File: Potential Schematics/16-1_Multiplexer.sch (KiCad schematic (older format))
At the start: 2 parts, among them U181 74LS04, U194 74LS04

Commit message: Adding Multiply Devide
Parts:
- U181, U194: symbol 74LS04 -> 4-bit_processor-rescue:74LS04
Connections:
- net 5:1_AND/b is gone; now on net 5:1_AND/b: U194.2
- net 5:1_AND/c is gone; now on net 5:1_AND/c: U181.13
- net 5:1_AND/b: no longer U194.1
- net 5:1_AND/c: no longer U181.12, U181.8
- new net 5:1_AND/b: U194.1
- new net 5:1_AND/c: U181.12, U181.8
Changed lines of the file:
@@
-EESchema Schematic File Version 2
-LIBS:power
-LIBS:device
-LIBS:switches
-LIBS:relays
-LIBS:motors
-LIBS:transistors
-LIBS:conn
-LIBS:linear
-LIBS:regul
-LIBS:74xx
-LIBS:cmos4000
-LIBS:adc-dac
-LIBS:memory
-LIBS:xilinx
-LIBS:microcontrollers
-LIBS:dsp
-LIBS:microchip
-LIBS:analog_switches
-LIBS:motorola
-LIBS:texas
-LIBS:intel
-LIBS:audio
-LIBS:interface
-LIBS:digital-audio
-LIBS:philips
-LIBS:display
-LIBS:cypress
-LIBS:siliconi
-LIBS:opto
-LIBS:atmel
-LIBS:contrib
-LIBS:valves
+EESchema Schematic File Version 4
 LIBS:4-bit_processor-cache
-EELAYER 25 0
+EELAYER 26 0
 EELAYER END
 $Descr A4 11693 8268
 encoding utf-8
-Sheet 378 449
+Sheet 378 451
 Title "16:1 Multiplexer"
 Date "2018-09-14"
@@
 $EndSheet
 $Comp
-L 74LS04 U194
+L 4-bit_processor-rescue:74LS04 U194
 U 1 1 5BB53D19
 P 1700 5450
@@
 $EndComp
 $Comp
-L 74LS04 U181
+L 4-bit_processor-rescue:74LS04 U181
 U 6 1 5BB54417
 P 1400 5450
@@
 $EndComp
 $Comp
-L 74LS04 U181
+L 4-bit_processor-rescue:74LS04 U181
 U 5 1 5BB55464
 P 1100 5450
@@
 $EndComp
 $Comp
-L 74LS04 U181
+L 4-bit_processor-rescue:74LS04 U181
 U 4 1 5BB5546A
 P 800 5450

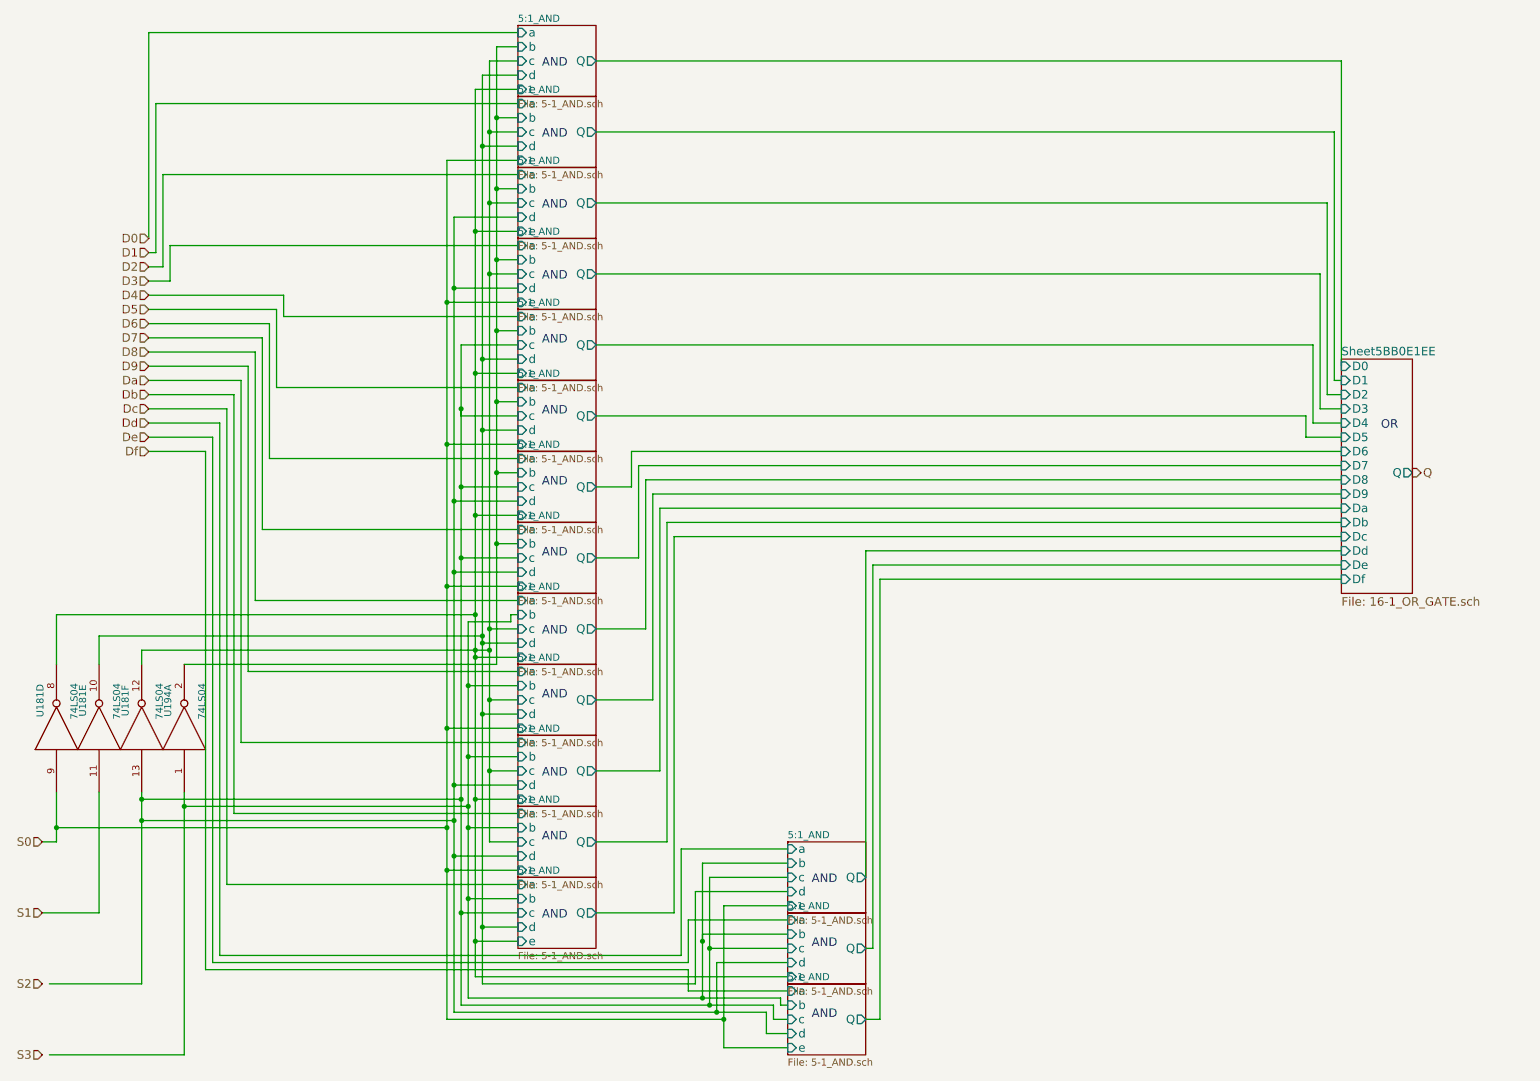
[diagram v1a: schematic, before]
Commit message: Finished PCB
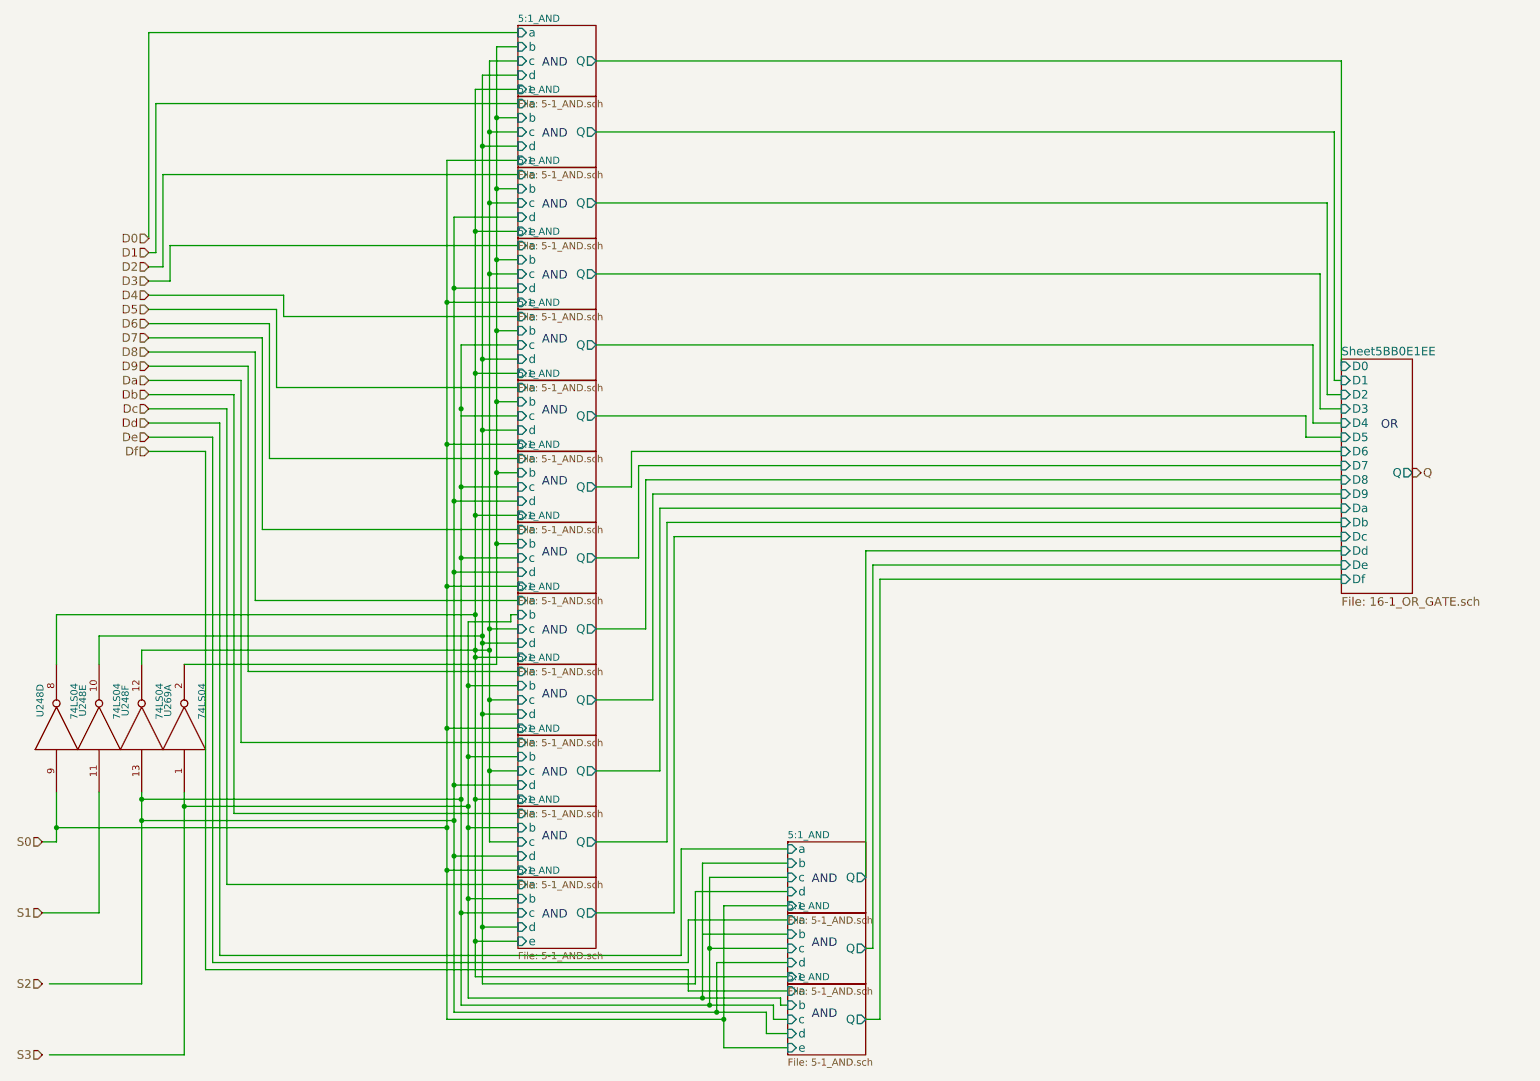
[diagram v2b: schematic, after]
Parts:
- U195: renamed from U181; footprint (none) -> Daniel_Kopp:DIP-14_300_ELL
- U208: renamed from U194; footprint (none) -> Daniel_Kopp:DIP-14_300_ELL
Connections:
- net 5:1_AND/b is gone; now on net 5:1_AND/b: U208.2
- net 5:1_AND/c is gone; now on net 5:1_AND/c: U195.13
- net 5:1_AND/b: no longer U208.1
- net 5:1_AND/c: no longer U195.12, U195.8
- new net 5:1_AND/b: U208.1
- new net 5:1_AND/c: U195.12, U195.8
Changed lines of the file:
@@
 $Descr A4 11693 8268
 encoding utf-8
-Sheet 378 451
+Sheet 378 456
 Title "16:1 Multiplexer"
 Date "2018-09-14"
@@
 $EndSheet
 $Comp
-L 4-bit_processor-rescue:74LS04 U194
+L 4-bit_processor-rescue:74LS04 U208
 U 1 1 5BB53D19
 P 1700 5450
-AR Path="/5B9D167A/5B9C0EA0/5BAE2F4B/5BAE3D50/5BB53D19" Ref="U194"  Part="1"
-AR Path="/5B9D167A/5B9C0EA0/5BAE2F4B/5BC8C0A9/5BB53D19" Ref="U194"  Part="5"
-AR Path="/5B9D167A/5B9C0EA0/5BAE2F4B/5BC8F4EC/5BB53D19" Ref="U233"  Part="3"
-AR Path="/5B9D167A/5B9C0EA0/5BAE2F4B/5BC8F503/5BB53D19" Ref="U253"  Part="1"
-F 0 "U194" H 1895 5565 50  0000 C CNN
+AR Path="/5B9D167A/5B9C0EA0/5BAE2F4B/5BAE3D50/5BB53D19" Ref="U208"  Part="1"
+AR Path="/5B9D167A/5B9C0EA0/5BAE2F4B/5BC8C0A9/5BB53D19" Ref="U208"  Part="5"
+AR Path="/5B9D167A/5B9C0EA0/5BAE2F4B/5BC8F4EC/5BB53D19" Ref="U248"  Part="3"
+AR Path="/5B9D167A/5B9C0EA0/5BAE2F4B/5BC8F503/5BB53D19" Ref="U269"  Part="1"
+F 0 "U269" H 1895 5565 50  0000 C CNN
 F 1 "74LS04" H 1890 5325 50  0000 C CNN
-F 2 "" H 1700 5450 50  0001 C CNN
+F 2 "Daniel_Kopp:DIP-14_300_ELL" H 1700 5450 50  0001 C CNN
 F 3 "" H 1700 5450 50  0001 C CNN
 	1    1700 5450
@@
 $EndComp
 $Comp
-L 4-bit_processor-rescue:74LS04 U181
+L 4-bit_processor-rescue:74LS04 U195
 U 6 1 5BB54417
 P 1400 5450
-AR Path="/5B9D167A/5B9C0EA0/5BAE2F4B/5BAE3D50/5BB54417" Ref="U181"  Part="6"
-AR Path="/5B9D167A/5B9C0EA0/5BAE2F4B/5BC8C0A9/5BB54417" Ref="U194"  Part="4"
-AR Path="/5B9D167A/5B9C0EA0/5BAE2F4B/5BC8F4EC/5BB54417" Ref="U233"  Part="2"
-AR Path="/5B9D167A/5B9C0EA0/5BAE2F4B/5BC8F503/5BB54417" Ref="U233"  Part="6"
-F 0 "U181" H 1595 5565 50  0000 C CNN
+AR Path="/5B9D167A/5B9C0EA0/5BAE2F4B/5BAE3D50/5BB54417" Ref="U195"  Part="6"
+AR Path="/5B9D167A/5B9C0EA0/5BAE2F4B/5BC8C0A9/5BB54417" Ref="U208"  Part="4"
+AR Path="/5B9D167A/5B9C0EA0/5BAE2F4B/5BC8F4EC/5BB54417" Ref="U248"  Part="2"
+AR Path="/5B9D167A/5B9C0EA0/5BAE2F4B/5BC8F503/5BB54417" Ref="U248"  Part="6"
+F 0 "U248" H 1595 5565 50  0000 C CNN
 F 1 "74LS04" H 1590 5325 50  0000 C CNN
-F 2 "" H 1400 5450 50  0001 C CNN
+F 2 "Daniel_Kopp:DIP-14_300_ELL" H 1400 5450 50  0001 C CNN
 F 3 "" H 1400 5450 50  0001 C CNN
 	6    1400 5450
@@
 $EndComp
 $Comp
-L 4-bit_processor-rescue:74LS04 U181
+L 4-bit_processor-rescue:74LS04 U195
 U 5 1 5BB55464
 P 1100 5450
-AR Path="/5B9D167A/5B9C0EA0/5BAE2F4B/5BAE3D50/5BB55464" Ref="U181"  Part="5"
-AR Path="/5B9D167A/5B9C0EA0/5BAE2F4B/5BC8C0A9/5BB55464" Ref="U194"  Part="3"
-AR Path="/5B9D167A/5B9C0EA0/5BAE2F4B/5BC8F4EC/5BB55464" Ref="U233"  Part="1"
-AR Path="/5B9D167A/5B9C0EA0/5BAE2F4B/5BC8F503/5BB55464" Ref="U233"  Part="5"
-F 0 "U181" H 1295 5565 50  0000 C CNN
+AR Path="/5B9D167A/5B9C0EA0/5BAE2F4B/5BAE3D50/5BB55464" Ref="U195"  Part="5"
+AR Path="/5B9D167A/5B9C0EA0/5BAE2F4B/5BC8C0A9/5BB55464" Ref="U208"  Part="3"
+AR Path="/5B9D167A/5B9C0EA0/5BAE2F4B/5BC8F4EC/5BB55464" Ref="U248"  Part="1"
+AR Path="/5B9D167A/5B9C0EA0/5BAE2F4B/5BC8F503/5BB55464" Ref="U248"  Part="5"
+F 0 "U248" H 1295 5565 50  0000 C CNN
 F 1 "74LS04" H 1290 5325 50  0000 C CNN
-F 2 "" H 1100 5450 50  0001 C CNN
+F 2 "Daniel_Kopp:DIP-14_300_ELL" H 1100 5450 50  0001 C CNN
 F 3 "" H 1100 5450 50  0001 C CNN
 	5    1100 5450
@@
 $EndComp
 $Comp
-L 4-bit_processor-rescue:74LS04 U181
+L 4-bit_processor-rescue:74LS04 U195
 U 4 1 5BB5546A
 P 800 5450
-AR Path="/5B9D167A/5B9C0EA0/5BAE2F4B/5BAE3D50/5BB5546A" Ref="U181"  Part="4"
-AR Path="/5B9D167A/5B9C0EA0/5BAE2F4B/5BC8C0A9/5BB5546A" Ref="U194"  Part="2"
-AR Path="/5B9D167A/5B9C0EA0/5BAE2F4B/5BC8F4EC/5BB5546A" Ref="U194"  Part="6"
-AR Path="/5B9D167A/5B9C0EA0/5BAE2F4B/5BC8F503/5BB5546A" Ref="U233"  Part="4"
-F 0 "U181" H 995 5565 50  0000 C CNN
+AR Path="/5B9D167A/5B9C0EA0/5BAE2F4B/5BAE3D50/5BB5546A" Ref="U195"  Part="4"
+AR Path="/5B9D167A/5B9C0EA0/5BAE2F4B/5BC8C0A9/5BB5546A" Ref="U208"  Part="2"
+AR Path="/5B9D167A/5B9C0EA0/5BAE2F4B/5BC8F4EC/5BB5546A" Ref="U208"  Part="6"
+AR Path="/5B9D167A/5B9C0EA0/5BAE2F4B/5BC8F503/5BB5546A" Ref="U248"  Part="4"
+F 0 "U248" H 995 5565 50  0000 C CNN
 F 1 "74LS04" H 990 5325 50  0000 C CNN
-F 2 "" H 800 5450 50  0001 C CNN
+F 2 "Daniel_Kopp:DIP-14_300_ELL" H 800 5450 50  0001 C CNN
 F 3 "" H 800 5450 50  0001 C CNN
 	4    800  5450
@@
 	700  6250 800  6250
 Wire Wire Line
-	800  6250 800  5900
+	800  6250 800  6150
 Wire Wire Line
 	700  6750 1100 6750
@@
 	750  7250 1400 7250
 Wire Wire Line
-	1400 7250 1400 5900
+	1400 7250 1400 6100
 Wire Wire Line
 	750  7750 1700 7750
 Wire Wire Line
-	1700 7750 1700 5900
+	1700 7750 1700 6000
 Wire Wire Line
 	1700 5000 3900 5000
 Wire Wire Line
-	3900 5000 3900 650
+	3900 5000 3900 4150
 Wire Wire Line
 	3900 650  4050 650
@@
 	1400 5000 1400 4900
 Wire Wire Line
-	1400 4900 3850 4900
-Wire Wire Line
-	3850 750  3850 6250
+	1400 4900 3750 4900
+Wire Wire Line
+	3850 750  3850 1250
 Wire Wire Line
 	3850 750  4050 750
@@
 	1100 4800 3800 4800
 Wire Wire Line
-	3800 850  3800 4850
+	3800 850  3800 1350
 Wire Wire Line
 	3800 850  4050 850
@@
 	800  4650 3750 4650
 Wire Wire Line
-	3750 950  3750 4950
+	3750 950  3750 1950
 Wire Wire Line
 	3750 950  4050 950
@@
 	4050 5350 3800 5350
 Wire Wire Line
-	3800 4800 3800 7250
+	3800 4800 3800 4850
 Wire Wire Line
 	3800 4850 4050 4850
@@
 	4050 5950 3750 5950
 Wire Wire Line
-	3750 4900 3750 7200
+	3750 4900 3750 4950
 Connection ~ 3750 4900
 Wire Wire Line
@@
 	1700 6000 3700 6000
 Wire Wire Line
-	3700 4700 3700 7350
+	3700 4700 3700 5150
 Wire Wire Line
 	3700 4700 4000 4700
@@
 	5950 6400 5350 6400
 Wire Wire Line
-	3700 7350 5900 7350
+	3700 7350 5350 7350
 Connection ~ 3700 6650
 Wire Wire Line
 	5950 6900 5350 6900
-Wire Wire Line
-	5350 6900 5350 6950
-Connection ~ 5350 6950
 Connection ~ 5350 7350
 Wire Wire Line
-	5350 6400 5350 7350
-Wire Wire Line
 	5900 7350 5900 7400
 Wire Wire Line
@@
 Wire Wire Line
 	1400 5950 3650 5950
-Wire Wire Line
-	3650 2750 3650 7400
 Wire Wire Line
 	3650 2750 4050 2750
@@
 Wire Wire Line
 	4050 3250 3650 3250
-Wire Wire Line
-	3650 3250 3650 3200
 Connection ~ 3650 3200
 Wire Wire Line
@@
 Connection ~ 3650 5950
 Wire Wire Line
-	3650 7400 5850 7400
-Wire Wire Line
-	5400 7400 5400 6500
+	3650 7400 5400 7400
+Wire Wire Line
+	5400 7400 5400 7000
 Wire Wire Line
 	5400 6500 5950 6500
@@
 	1400 6100 3600 6100
 Wire Wire Line
-	3600 1850 3600 7450
+	3600 1850 3600 2350
 Wire Wire Line
 	3600 1850 4050 1850
@@
 Connection ~ 3600 6100
 Wire Wire Line
-	3600 7450 5800 7450
+	3600 7450 5450 7450
 Wire Wire Line
 	5450 7450 5450 7100
@@
 	800  6150 3550 6150
 Wire Wire Line
-	3550 1450 3550 7500
+	3550 1450 3550 2450
 Wire Wire Line
 	3550 1450 4050 1450
@@
 	3550 7500 5500 7500
 Wire Wire Line
-	5500 6700 5500 7700
+	5500 6700 5500 7500
 Wire Wire Line
 	5500 7700 5950 7700
@@
 Text Notes 6300 7500 2    60   ~ 0
 AND
+Wire Wire Line
+	3750 1950 3750 2950
+Wire Wire Line
+	3900 1150 3900 650
+Wire Wire Line
+	3850 1250 3850 1750
+Wire Wire Line
+	3800 1350 3800 2850
+Wire Wire Line
+	3900 1650 3900 1150
+Wire Wire Line
+	3850 1750 3850 2250
+Wire Wire Line
+	3850 2250 3850 4750
+Wire Wire Line
+	3900 2150 3900 1650
+Wire Wire Line
+	3900 2650 3900 2150
+Wire Wire Line
+	3750 2950 3750 3950
+Wire Wire Line
+	3800 3350 3800 4800
+Wire Wire Line
+	3800 2850 3800 3350
+Wire Wire Line
+	3900 3150 3900 2650
+Wire Wire Line
+	3750 3950 3750 4650
+Wire Wire Line
+	3900 3650 3900 3150
+Wire Wire Line
+	3900 4150 3900 3650
+Wire Wire Line
+	3850 4750 3850 4900
+Wire Wire Line
+	3750 4650 3750 4900
+Wire Wire Line
+	3850 4900 3850 5250
+Wire Wire Line
+	3800 4850 3800 5350
+Wire Wire Line
+	3850 5250 3850 5750
+Wire Wire Line
+	3750 4900 3850 4900
+Wire Wire Line
+	3750 4950 3750 5950
+Wire Wire Line
+	3800 5350 3800 6850
+Wire Wire Line
+	3750 5950 3750 6950
+Wire Wire Line
+	3850 5750 3850 6250
+Wire Wire Line
+	3750 6950 3750 7200
+Wire Wire Line
+	3800 6850 3800 7250
+Wire Wire Line
+	1700 6000 1700 5900
+Wire Wire Line
+	3700 5150 3700 5650
+Wire Wire Line
+	3700 5650 3700 6000
+Wire Wire Line
+	3700 6000 3700 6150
+Wire Wire Line
+	3700 6150 3700 6650
+Wire Wire Line
+	3700 6650 3700 7350
+Wire Wire Line
+	5350 7350 5900 7350
+Wire Wire Line
+	1400 5950 1400 5900
+Wire Wire Line
+	3650 3750 3650 4250
+Wire Wire Line
+	3650 4250 3650 5950
+Wire Wire Line
+	3650 5950 3650 6750
+Wire Wire Line
+	3650 6750 3650 7400
+Wire Wire Line
+	5400 7000 5400 6500
+Wire Wire Line
+	5400 7400 5850 7400
+Wire Wire Line
+	1400 6100 1400 5950
+Wire Wire Line
+	3600 2350 3600 3850
+Wire Wire Line
+	3600 3850 3600 4350
+Wire Wire Line
+	3600 4350 3600 5850
+Wire Wire Line
+	3600 5850 3600 6100
+Wire Wire Line
+	3600 6100 3600 6350
+Wire Wire Line
+	3600 6350 3600 7450
+Wire Wire Line
+	5450 7450 5800 7450
+Wire Wire Line
+	800  6150 800  5900
+Wire Wire Line
+	3550 2450 3550 3450
+Wire Wire Line
+	3550 3450 3550 4450
+Wire Wire Line
+	3550 4450 3550 5450
+Wire Wire Line
+	3550 5450 3550 6150
+Wire Wire Line
+	3550 6150 3550 6450
+Wire Wire Line
+	3550 6450 3550 7500
+Wire Wire Line
+	5500 7500 5500 7700
+Wire Wire Line
+	5350 6400 5350 7350
+Wire Wire Line
+	3650 2750 3650 3750
 $EndSCHEMATC
